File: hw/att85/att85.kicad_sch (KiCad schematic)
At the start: 42 parts, among them J101 Barrel_Jack_Switch, J102 Screw_Terminal_01x03, J103 AVR-ISP-6, J104 Conn_01x02, J105 Conn_01x02, Q101 BC817, SW101 SW_Push, SW102 SW_Push, SW103 SW_Push, SW104 SW_Push, SW105 SW_Push, SW106 SW_Push, U101 ATtiny85-20P, U102 MT3608-MODULE, U105 74AHC1G125

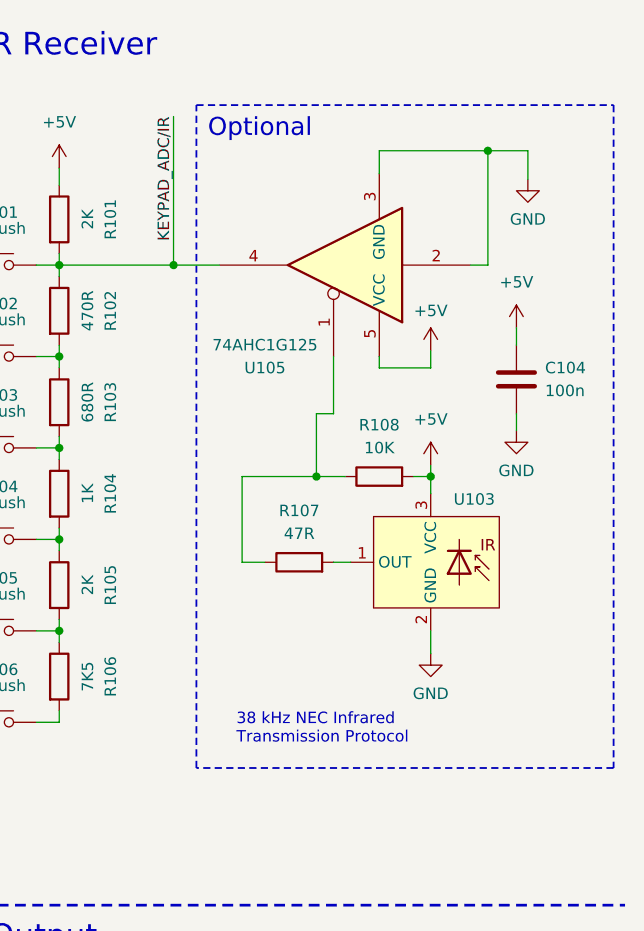
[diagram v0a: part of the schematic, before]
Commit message: chore(hw): add notes
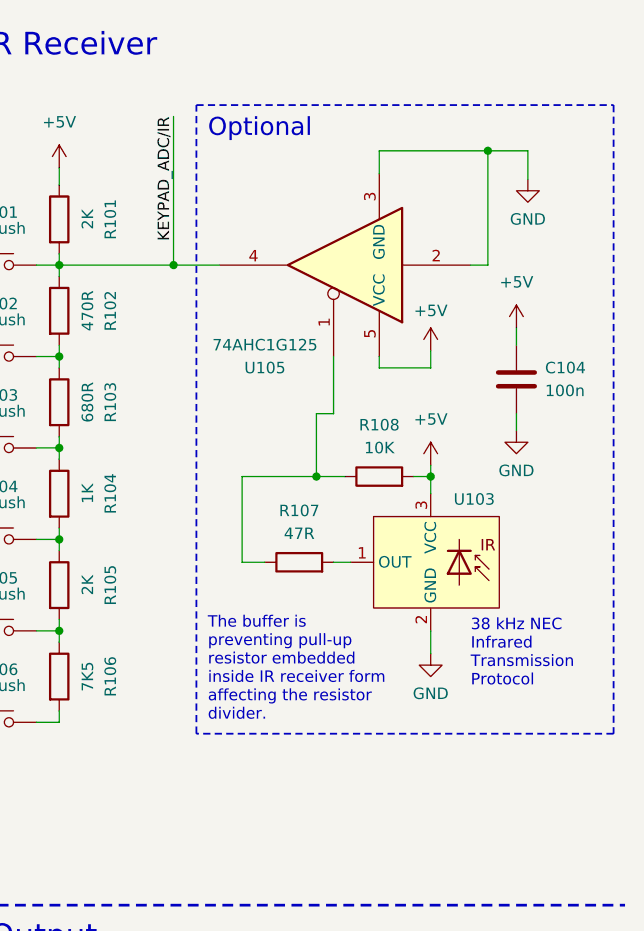
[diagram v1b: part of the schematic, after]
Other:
- note added: "The buffer is preventing pull-up resistor embedded inside IR receiver form affecting the resistor divider."
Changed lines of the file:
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@@
     (stroke (width 0.3) (type dash))
   )
-  (rectangle (start 236.855 22.225) (end 283.21 95.885)
+  (rectangle (start 236.855 22.225) (end 283.21 92.075)
     (stroke (width 0.2) (type dash))
     (fill (type none))
@@
   (text "RIGHT" (at 205.74 80.645 0)
     (effects (font (size 1.27 1.27)) (justify right bottom))
+  )
+  (text "The buffer is\npreventing pull-up\nresistor embedded\ninside IR receiver form\naffecting the resistor\ndivider."
+    (at 238.125 90.805 0)
+    (effects (font (size 1.27 1.27)) (justify left bottom))
   )
   (text "Battery Power (Optional)" (at 13.97 64.77 0)
@@
     (effects (font (size 1.27 1.27)) (justify right bottom))
   )
-  (text "38 kHz NEC Infrared\nTransmission Protocol" (at 241.3 93.345 0)
+  (text "38 kHz NEC\nInfrared\nTransmission\nProtocol" (at 267.335 86.995 0)
     (effects (font (size 1.27 1.27)) (justify left bottom))
   )
